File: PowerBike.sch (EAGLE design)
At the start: 2 parts

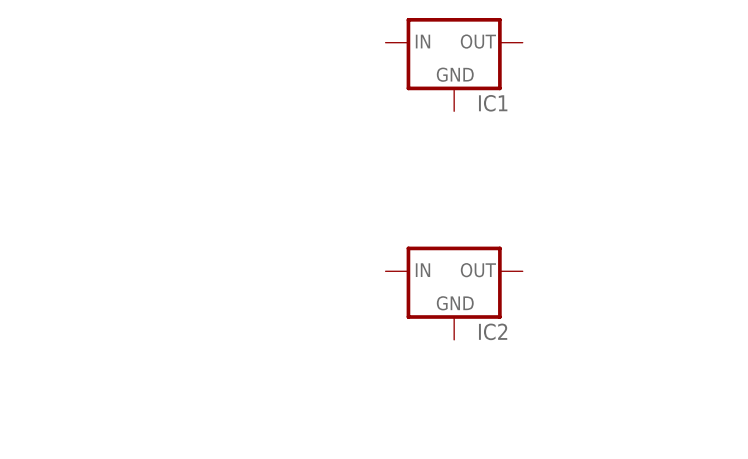
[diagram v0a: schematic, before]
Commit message: Schematic almost ready
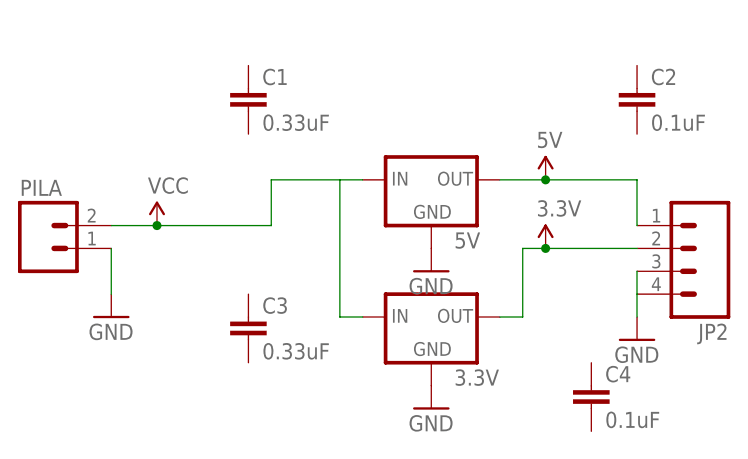
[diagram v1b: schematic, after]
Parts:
- removed IC1, IC2: (no value), SparkFun-PowerIC:V_REG_78XXSIDE
- added 3.3V, 5V: (no value), SparkFun-PowerIC:V_REG_78XXSIDE
- added C1, C3: 0.33uF, SparkFun-Passives:CAP0603-CAP
- added C2, C4: 0.1uF, SparkFun-Passives:CAP0603-CAP
- added JP2: (no value), SparkFun-Connectors:M04LOCK_LONGPADS
- added PILA: (no value), SparkFun-Connectors:M02LOCK_LONGPADS
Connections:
- new net 3.3V: 3.3V.OUT, JP2.2
- new net 5V: 5V.OUT, JP2.1
- new net GND: 3.3V.GND, 5V.GND, JP2.3, JP2.4, PILA.1
- new net VCC: 3.3V.IN, 5V.IN, PILA.2
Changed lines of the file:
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@@
 <?xml version="1.0" encoding="utf-8"?>
 <!DOCTYPE eagle SYSTEM "eagle.dtd">
-<eagle version="6.2">
+<eagle version="6.3">
 <drawing>
 <settings>
@@
 <layer number="144" name="Drill_legend" color="7" fill="1" visible="no" active="yes"/>
 <layer number="151" name="HeatSink" color="7" fill="1" visible="no" active="yes"/>
+<layer number="199" name="Contour" color="7" fill="1" visible="yes" active="yes"/>
 <layer number="200" name="200bmp" color="1" fill="10" visible="no" active="yes"/>
 <layer number="201" name="201bmp" color="2" fill="10" visible="no" active="yes"/>
@@
 </classes>
 <parts>
-<part name="IC1" library="SparkFun-PowerIC" deviceset="V_REG_78XX" device="SIDE"/>
-<part name="IC2" library="SparkFun-PowerIC" deviceset="V_REG_78XX" device="SIDE"/>
+<part name="5V" library="SparkFun-PowerIC" deviceset="V_REG_78XX" device="SIDE"/>
+<part name="3.3V" library="SparkFun-PowerIC" deviceset="V_REG_78XX" device="SIDE"/>
+<part name="C1" library="SparkFun-Passives" deviceset="CAP" device="0603-CAP" value="0.33uF"/>
+<part name="C2" library="SparkFun-Passives" deviceset="CAP" device="0603-CAP" value="0.1uF"/>
+<part name="C3" library="SparkFun-Passives" deviceset="CAP" device="0603-CAP" value="0.33uF"/>
+<part name="C4" library="SparkFun-Passives" deviceset="CAP" device="0603-CAP" value="0.1uF"/>
+<part name="PILA" library="SparkFun-Connectors" deviceset="M02" device="LOCK_LONGPADS"/>
+<part name="JP2" library="SparkFun-Connectors" deviceset="M04" device="LOCK_LONGPADS"/>
+<part name="P+1" library="SparkFun-Aesthetics" deviceset="3.3V" device=""/>
+<part name="U$1" library="SparkFun-Aesthetics" deviceset="5V" device=""/>
+<part name="GND1" library="SparkFun-Aesthetics" deviceset="GND" device=""/>
+<part name="P+2" library="SparkFun-Aesthetics" deviceset="VCC" device=""/>
+<part name="GND2" library="SparkFun-Aesthetics" deviceset="GND" device=""/>
+<part name="GND3" library="SparkFun-Aesthetics" deviceset="GND" device=""/>
+<part name="GND4" library="SparkFun-Aesthetics" deviceset="GND" device=""/>
 </parts>
 <sheets>
@@
 </plain>
 <instances>
-<instance part="IC1" gate="G$1" x="7.62" y="73.66"/>
-<instance part="IC2" gate="G$1" x="7.62" y="48.26"/>
+<instance part="5V" gate="G$1" x="5.08" y="58.42"/>
+<instance part="3.3V" gate="G$1" x="5.08" y="43.18"/>
+<instance part="C1" gate="G$1" x="-15.24" y="66.04"/>
+<instance part="C2" gate="G$1" x="27.94" y="66.04"/>
+<instance part="C3" gate="G$1" x="-15.24" y="40.64"/>
+<instance part="C4" gate="G$1" x="22.86" y="33.02"/>
+<instance part="PILA" gate="G$1" x="-38.1" y="50.8"/>
+<instance part="JP2" gate="G$1" x="33.02" y="50.8" rot="R180"/>
+<instance part="P+1" gate="G$1" x="17.78" y="50.8"/>
+<instance part="U$1" gate="G$1" x="17.78" y="58.42"/>
+<instance part="GND1" gate="1" x="-30.48" y="43.18"/>
+<instance part="P+2" gate="1" x="-25.4" y="53.34"/>
+<instance part="GND2" gate="1" x="5.08" y="33.02"/>
+<instance part="GND3" gate="1" x="5.08" y="48.26"/>
+<instance part="GND4" gate="1" x="27.94" y="40.64"/>
 </instances>
 <busses>
 </busses>
 <nets>
+<net name="GND" class="0">
+<segment>
+<pinref part="PILA" gate="G$1" pin="1"/>
+<pinref part="GND1" gate="1" pin="GND"/>
+<wire x1="-30.48" y1="50.8" x2="-30.48" y2="45.72" width="0.1524" layer="91"/>
+</segment>
+<segment>
+<pinref part="3.3V" gate="G$1" pin="GND"/>
+<pinref part="GND2" gate="1" pin="GND"/>
+</segment>
+<segment>
+<pinref part="5V" gate="G$1" pin="GND"/>
+<pinref part="GND3" gate="1" pin="GND"/>
+</segment>
+<segment>
+<pinref part="GND4" gate="1" pin="GND"/>
+<pinref part="JP2" gate="G$1" pin="4"/>
+<wire x1="27.94" y1="43.18" x2="27.94" y2="45.72" width="0.1524" layer="91"/>
+<pinref part="JP2" gate="G$1" pin="3"/>
+<wire x1="27.94" y1="45.72" x2="27.94" y2="48.26" width="0.1524" layer="91"/>
+</segment>
+</net>
+<net name="5V" class="0">
+<segment>
+<pinref part="5V" gate="G$1" pin="OUT"/>
+<wire x1="12.7" y1="58.42" x2="17.78" y2="58.42" width="0.1524" layer="91"/>
+<pinref part="JP2" gate="G$1" pin="1"/>
+<wire x1="17.78" y1="58.42" x2="27.94" y2="58.42" width="0.1524" layer="91"/>
+<wire x1="27.94" y1="58.42" x2="27.94" y2="53.34" width="0.1524" layer="91"/>
+<pinref part="U$1" gate="G$1" pin="5V"/>
+<junction x="17.78" y="58.42"/>
+</segment>
+</net>
+<net name="3.3V" class="0">
+<segment>
+<pinref part="3.3V" gate="G$1" pin="OUT"/>
+<wire x1="12.7" y1="43.18" x2="15.24" y2="43.18" width="0.1524" layer="91"/>
+<wire x1="15.24" y1="43.18" x2="15.24" y2="50.8" width="0.1524" layer="91"/>
+<pinref part="JP2" gate="G$1" pin="2"/>
+<wire x1="15.24" y1="50.8" x2="17.78" y2="50.8" width="0.1524" layer="91"/>
+<pinref part="P+1" gate="G$1" pin="3.3V"/>
+<wire x1="17.78" y1="50.8" x2="27.94" y2="50.8" width="0.1524" layer="91"/>
+<junction x="17.78" y="50.8"/>
+</segment>
+</net>
+<net name="VCC" class="0">
+<segment>
+<pinref part="PILA" gate="G$1" pin="2"/>
+<wire x1="-30.48" y1="53.34" x2="-25.4" y2="53.34" width="0.1524" layer="91"/>
+<wire x1="-25.4" y1="53.34" x2="-12.7" y2="53.34" width="0.1524" layer="91"/>
+<wire x1="-12.7" y1="53.34" x2="-12.7" y2="58.42" width="0.1524" layer="91"/>
+<pinref part="5V" gate="G$1" pin="IN"/>
+<wire x1="-12.7" y1="58.42" x2="-5.08" y2="58.42" width="0.1524" layer="91"/>
+<pinref part="3.3V" gate="G$1" pin="IN"/>
+<wire x1="-5.08" y1="58.42" x2="-2.54" y2="58.42" width="0.1524" layer="91"/>
+<wire x1="-2.54" y1="43.18" x2="-5.08" y2="43.18" width="0.1524" layer="91"/>
+<wire x1="-5.08" y1="43.18" x2="-5.08" y2="58.42" width="0.1524" layer="91"/>
+<pinref part="P+2" gate="1" pin="VCC"/>
+<junction x="-25.4" y="53.34"/>
+</segment>
+</net>
 </nets>
 </sheet>
